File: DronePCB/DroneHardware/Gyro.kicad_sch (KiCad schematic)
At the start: 5 parts, among them U301 MPU-6050

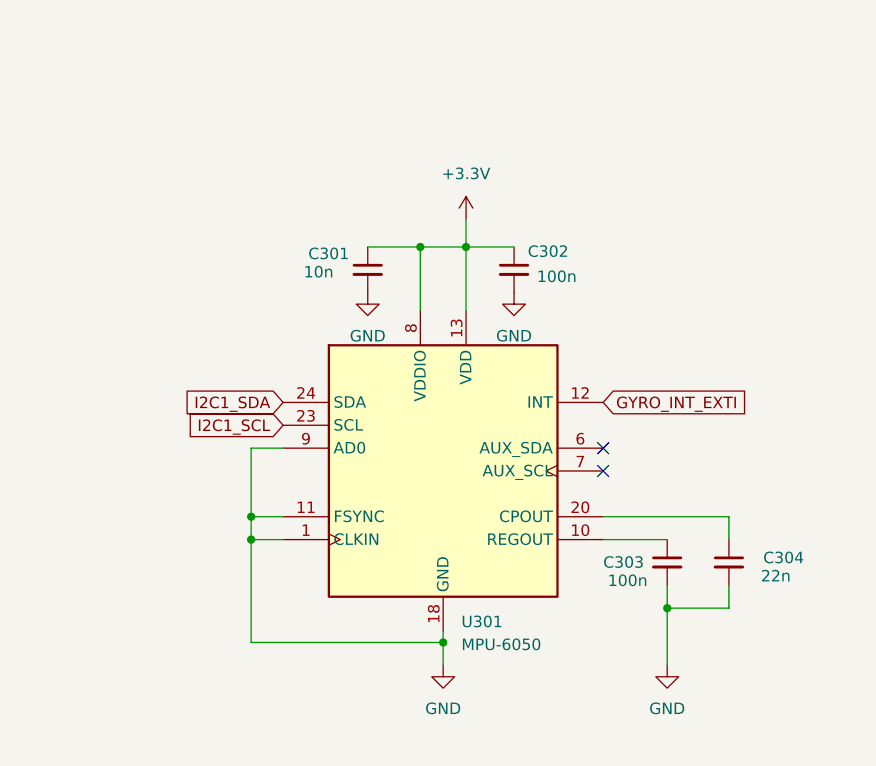
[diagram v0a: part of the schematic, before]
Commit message: Utilizzo di mpu-6000
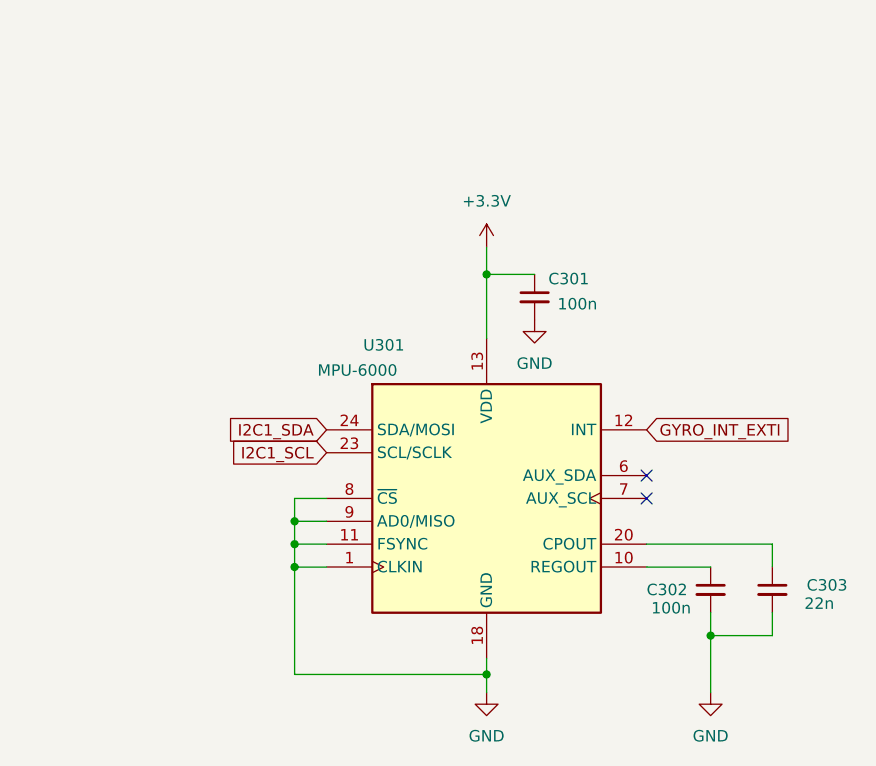
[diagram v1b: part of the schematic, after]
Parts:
- removed C304: 22n, Capacitor_SMD:C_0402_1005Metric, symbol Device:C_Small
- removed U301: MPU-6050, Sensor_Motion:InvenSense_QFN-24_4x4mm_P0.5mm, symbol Sensor_Motion:MPU-6050
- added U301: MPU-6000, Sensor_Motion:InvenSense_QFN-24_4x4mm_P0.5mm, symbol Sensor_Motion:MPU-6000
- C301: value 10n -> 100n
- C303: value 100n -> 22n
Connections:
- net +3V3: now also U301.13 (VDD); no longer C302.1
- net GND: now also U301.1 (CLKIN), U301.11 (FSYNC), U301.18 (GND), U301.8 (~{CS}), U301.9 (AD0/MISO)
- net GYRO_INT_EXTI: now also U301.12 (INT)
- net I2C1_SCL: now also U301.23 (SCL/SCLK)
- net I2C1_SDA: now also U301.24 (SDA/MOSI)
- net at C303.1: now also U301.20 (CPOUT)
- new net: C302.1, U301.10 (REGOUT)
